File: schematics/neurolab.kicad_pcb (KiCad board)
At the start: 2 copper layers, 124.9 x 52.5 mm, 173 parts, among them J1 GS3, J10 GS3, J11 GS2, J12 GS3, J13 GS3, J14 GS3, J15 GS3, J16 Channel, J17 External, J18 USB_OTG, J19 GS3, J2 GS3, J20 GS2, J21 GS2, J22 GS2, J23 GS2, J24 GS2, J25 GS2, J26 ICSP Port, J27 GS2, J28 GS2, J29 Teensy Port, J3 GS3, J30 GS3, J31 GS3, J32 Bluetooth, J33 Reset Select, J34 GS2, J35 High Power, J36 12 Volts, J4 GS2, J5 GS2, J6 GS3, J7 GS3, J8 GS2, J9 GS3, Q1 2N7002, U1 ADP1720ARMZ-5, U10 OPA2111KP, U11 AD8422ARMZ, U12 OP4117, U13 OPA2111KP, U14 AD8422ARMZ, U15 OP4117, U16 AD7173, U17 ADR445BR, U18 Arduino, U2 ADP1720ARMZ-3.3, U3 AD8475, U4 AD8475, U5 MAX7480ESA+, U6 MAX7480ESA+, U7 MAX7480ESA+, U8 MAX7480ESA+, U9 TLC555CD, Y1 FA-20H

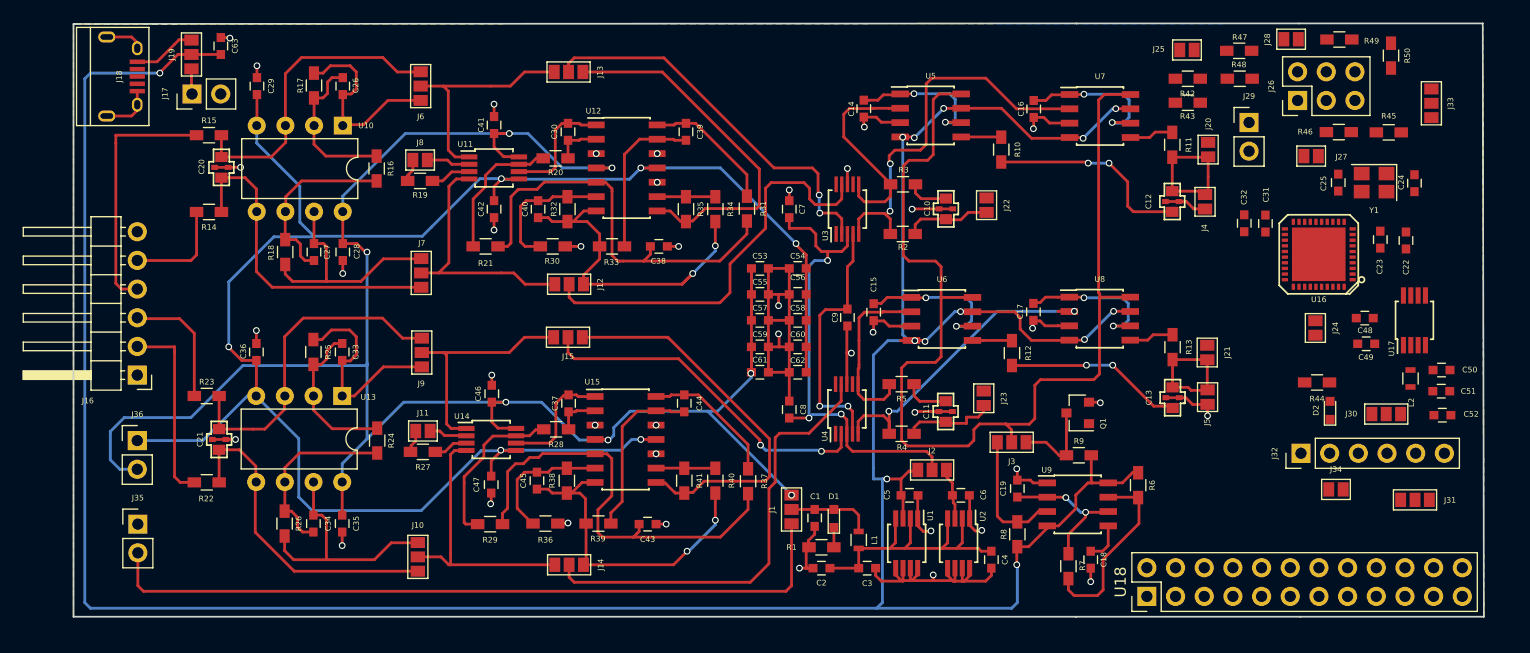
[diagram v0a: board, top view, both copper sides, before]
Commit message: refactor: route improvements
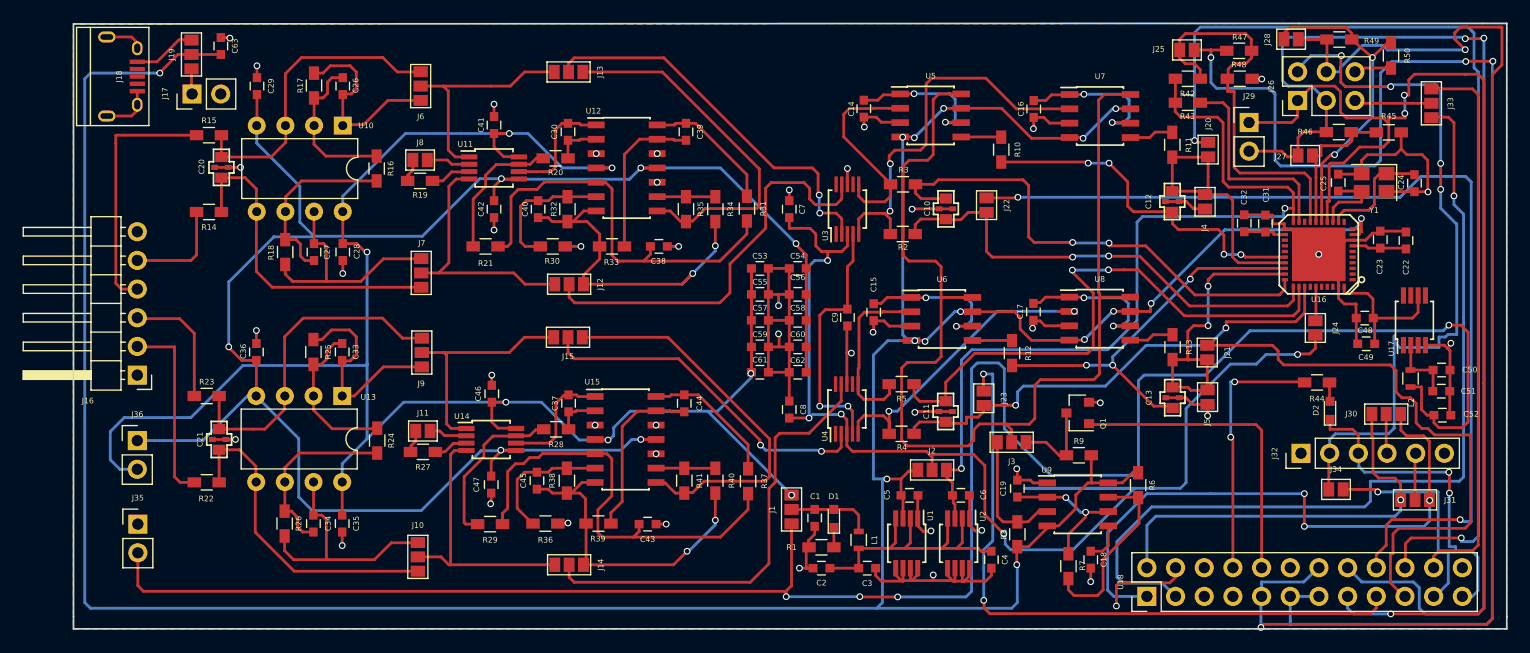
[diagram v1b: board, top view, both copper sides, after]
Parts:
- moved J27 0.53 mm to (199.2, 84.0)
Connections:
- J31 pad 1: TxO -> RxI
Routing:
- net CS: track 0.00 -> 118.3 mm, vias 0 -> 3
- net +5.5V: track 66.7 -> 181.8 mm, vias 0 -> 4
- net MISO: track 0.00 -> 108.9 mm, vias 0 -> 2
- net SCL: track 0.00 -> 104.0 mm, vias 0 -> 2
- net MOSI: track 0.00 -> 103.3 mm, vias 0 -> 3
- net GND: track 139.5 -> 235.5 mm, vias 40 -> 47
- net AD3: track 0.00 -> 90.2 mm, vias 0 -> 2
- net AD1: track 0.00 -> 86.1 mm, vias 0 -> 2
- net Net-(J33-Pad1): track 0.00 -> 80.7 mm, vias 0 -> 1
- net +3V: track 4.67 -> 78.3 mm, vias 0 -> 2
- net VCCIO: track 41.9 -> 114.7 mm, vias 3 -> 5
- net VCC: track 0.00 -> 64.9 mm, vias 0 -> 4
- net AD0: track 0.00 -> 59.6 mm, vias 0 -> 2
- net TxO: track 0.00 -> 53.3 mm, vias 0 -> 3
- net AD2: track 0.00 -> 50.6 mm
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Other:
- board size 124.9 x 52.5 mm -> 127 x 53.6 mm
- net class Default: clearance 0.2 -> 0.1
- rule trace_clearance: 0.2 -> 0.1
- rule trace_min: 0.2 -> 0.1
- rule via_min_size: 0.4 -> 0.3

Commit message: optimize: routing and placement
optimize: squeeze space

optimize: squeeze space contd.

optimize: contd.
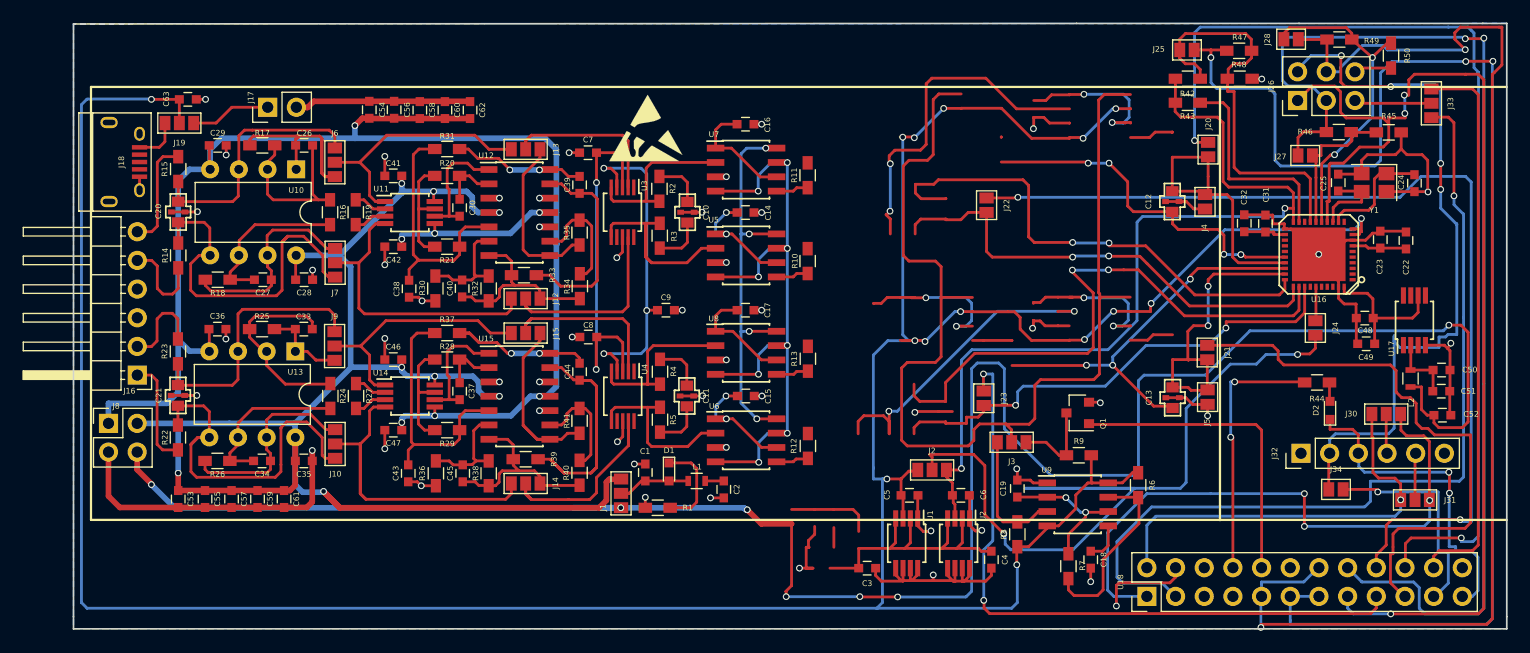
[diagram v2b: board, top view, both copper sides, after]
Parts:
- removed J11: GS2, Connectors:GS2
- removed J29: Teensy Port, Pin_Headers:Pin_Header_Straight_1x02_Pitch2.54mm
- removed J35: High Power, Pin_Headers:Pin_Header_Straight_1x02_Pitch2.54mm
- removed J36: 12 Volts, Pin_Headers:Pin_Header_Straight_1x02_Pitch2.54mm
- added REF***: ESD-Logo_6.6x6mm_SilkScreen, Symbols:ESD-Logo_6.6x6mm_SilkScreen, F.Cu at (140.8, 81.5)
- J8: value GS2 -> PowerOut; footprint Connectors:GS2 -> Pin_Headers:Pin_Header_Straight_2x02_Pitch2.54mm
- moved C53 55.4 mm to (99.3, 114.4), turned to 270 degrees
- moved C55 52.4 mm to (101.7, 114.4), turned to 270 degrees
- moved C57 49.4 mm to (104.0, 114.4), turned to 270 degrees
- moved C59 46.5 mm to (106.3, 114.4), turned to 270 degrees
- moved C61 43.6 mm to (108.7, 114.4), turned to 270 degrees
- moved C54 40.5 mm to (116.2, 79.9), turned to 270 degrees
- moved C56 39.3 mm to (118.5, 79.9), turned to 270 degrees
- moved C58 38.3 mm to (120.7, 79.9), turned to 270 degrees
- moved C60 37.6 mm to (123.0, 79.9), turned to 270 degrees
- moved C62 37.2 mm to (125.2, 79.9), turned to 270 degrees
- moved J8 36.1 mm to (93.2, 107.7), turned to 0 degrees
- moved R11 32.4 mm to (155.1, 85.7), turned to 90 degrees
- moved R13 32.3 mm to (155.1, 102.0), turned to 90 degrees
- moved U7 31.7 mm to (149.6, 85.2)
- moved U8 31.5 mm to (149.6, 101.4)
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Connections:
- J16 pad 1: GND -> /Amplifier Block 2/IN+
- J16 pad 2: /Amplifier Block 2/IN+ -> /Amplifier Block 2/IN-
- J16 pad 3: /Amplifier Block 2/IN- -> GND
- J16 pad 4: /Amplifier Block 1/IN- -> GND
- J16 pad 6: GND -> /Amplifier Block 1/IN-
- J8 pad 1: Net-(J8-Pad1) -> -12V
- J8 pad 2: Net-(J8-Pad2) -> +12V
- R19 pad 2: Net-(J8-Pad1) -> Net-(R19-Pad2)
- R27 pad 2: Net-(J11-Pad1) -> Net-(R27-Pad2)
- U11 pad 2: Net-(J8-Pad2) -> Net-(R19-Pad2)
- U14 pad 2: Net-(J11-Pad2) -> Net-(R27-Pad2)
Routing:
- net (no net): track 0.00 -> 140.0 mm, vias 0 -> 14
- net +5V: track 294.6 -> 352.0 mm, vias 15 -> 23
- net /Clock Block/CLK: track 98.2 -> 134.0 mm, vias 0 -> 4
- net /Attenuator/+OUTA: track 34.5 -> 14.7 mm, vias 2 -> 0
- net /Attenuator/+IN0.4XA: track 36.4 -> 17.7 mm
- net /Attenuator/-IN0.4XA: track 34.5 -> 15.8 mm, vias 2 -> 0
- net /Attenuator/+IN0.4XB: track 39.7 -> 21.3 mm
- net Net-(J13-Pad3): track 32.5 -> 15.1 mm
- net Net-(J15-Pad3): track 34.9 -> 18.4 mm
- net Net-(C43-Pad1): track 39.2 -> 22.8 mm
- net /Attenuator/-IN0.4XB: track 30.8 -> 15.9 mm, vias 2 -> 0
- net /Attenuator/+OUTB: track 28.9 -> 14.5 mm, vias 2 -> 0
- net Net-(C38-Pad1): track 36.9 -> 22.5 mm
- net Net-(C40-Pad1): track 31.2 -> 16.9 mm, vias 2 -> 0
- net Net-(C44-Pad1): track 15.2 -> 29.4 mm
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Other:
- net class Default: clearance 0.1 -> 0.16
- rule trace_clearance: 0.1 -> 0.16
- rule trace_min: 0.1 -> 0.16
